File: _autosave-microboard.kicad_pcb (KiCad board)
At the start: 2 copper layers, 95 parts, among them J1 Conn_01x01, J10 Conn_01x01, J11 Conn_01x01, J12 Conn_01x10, J13 Conn_01x01, J17 Conn_01x01, J18 Conn_01x01, J2 Conn_01x10, J21 Conn_01x01_Socket, J22 Conn_01x01_Socket, J24 Conn_01x01, J25 Conn_01x01, J3 Conn_02x12, J39 Conn_01x10, J4 USB_C_Receptacle_USB2.0, J40 Conn_01x10, J41 Conn_01x10, J43 Conn_01x05, J44 Conn_01x09, J45 Conn_01x08, J5 Conn_01x04, J6 Conn_01x04, J7 Conn_01x05, J8 Conn_01x10, J9 Conn_01x01, SW1 SW_Push, SW3 SW_Push, SW4 SW_Push, SW7 RotaryEncoder_Switch, U1 USBLC6-2SC6, U2 ATSAMD21G18A-AUT, U3 LF33_TO220, U4 TXS0108EPW, U7 LF50_TO220, Y1 32768Hz

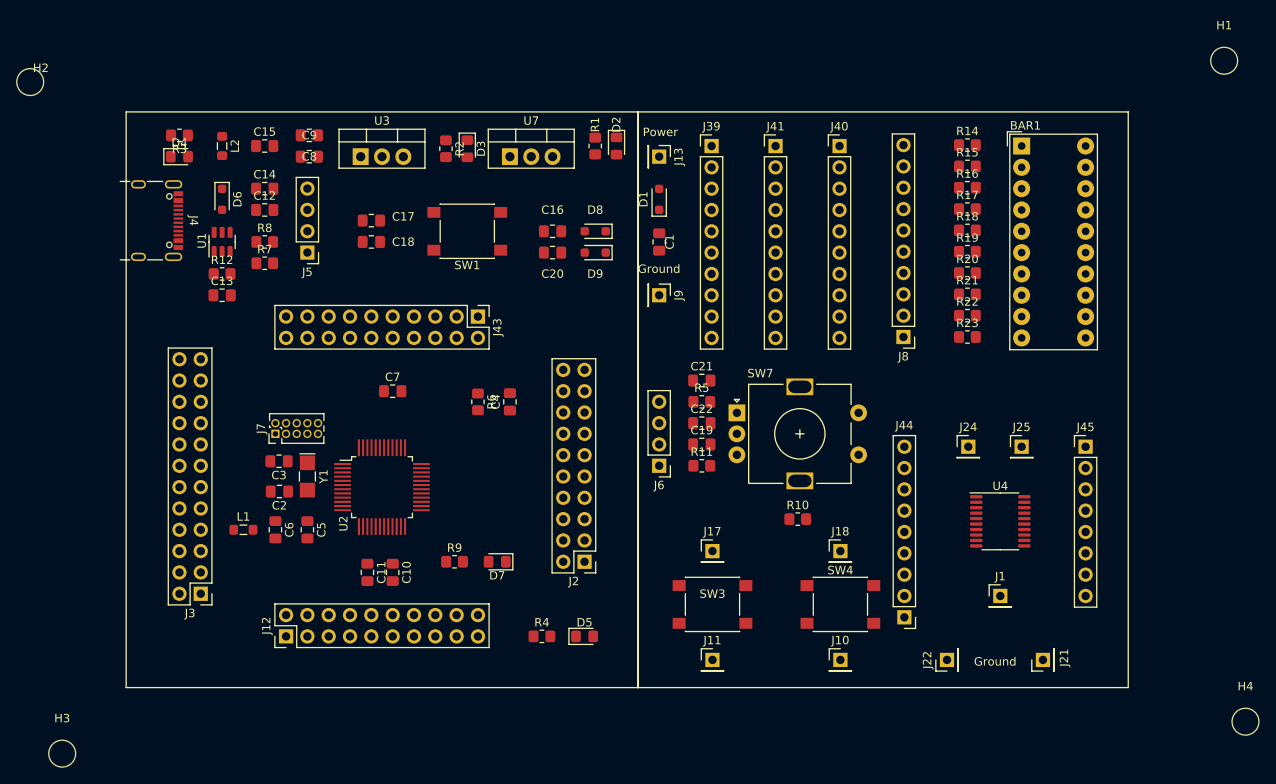
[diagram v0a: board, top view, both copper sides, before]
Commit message: updated
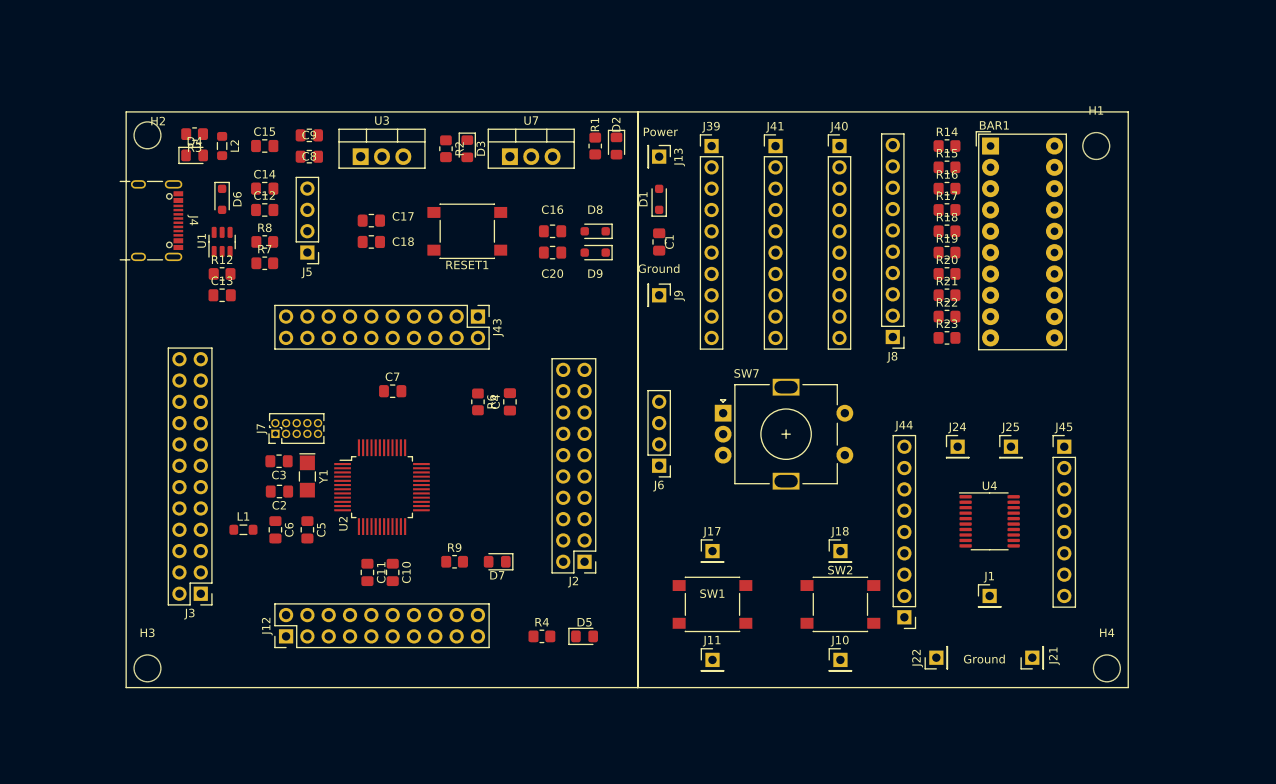
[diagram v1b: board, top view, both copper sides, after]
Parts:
- removed C19, C21, C22: 0.1uF, Capacitor_SMD:C_0805_2012Metric_Pad1.18x1.45mm_HandSolder
- removed R10, R11, R5: 22K, Resistor_SMD:R_0805_2012Metric_Pad1.20x1.40mm_HandSolder
- moved H1 18.3 mm to (242.6, 59.7)
- moved H4 17.7 mm to (243.8, 121.9)
- moved H2 15.3 mm to (129.5, 58.4)
- moved H3 14.4 mm to (129.5, 121.9)
- moved BAR1 3.70 mm to (230.0, 59.7)
- moved J45 2.54 mm to (238.8, 95.5)
- moved R14 2.43 mm to (224.8, 59.7)
- moved R15 2.43 mm to (224.8, 62.2)
- moved R16 2.43 mm to (224.8, 64.8)
- moved R17 2.43 mm to (224.8, 67.3)
- moved R19 2.43 mm to (224.8, 72.4)
- moved R20 2.43 mm to (224.8, 74.9)
- moved R21 2.43 mm to (224.8, 77.5)
- moved R22 2.43 mm to (224.8, 80.0)
- moved R23 2.43 mm to (224.8, 82.5)
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- renumbered SW1 to RESET1, SW3 to SW1, SW4 to SW2
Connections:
- J12 pad 10: GND -> Net-(J12-Pin_10)
- J12 pad 11: +3.3V -> Net-(J12-Pin_11)
- J12 pad 12: Net-(J12-Pin_12) -> Net-(J12-Pin_11)
- J12 pad 14: Net-(J12-Pin_14) -> Net-(J12-Pin_13)
- J12 pad 16: Net-(J12-Pin_16) -> Net-(J12-Pin_15)
- J12 pad 18: Net-(J12-Pin_18) -> Net-(J12-Pin_17)
- J12 pad 19: Net-(J12-Pin_19) -> GND
- J12 pad 2: Net-(J12-Pin_12) -> +3.3V
- J12 pad 3: Net-(J12-Pin_13) -> Net-(J12-Pin_3)
- J12 pad 4: Net-(J12-Pin_14) -> Net-(J12-Pin_3)
- J12 pad 5: Net-(J12-Pin_15) -> Net-(J12-Pin_5)
- J12 pad 6: Net-(J12-Pin_16) -> Net-(J12-Pin_5)
- J12 pad 7: Net-(J12-Pin_17) -> Net-(J12-Pin_7)
- J12 pad 8: Net-(J12-Pin_18) -> Net-(J12-Pin_7)
- J12 pad 9: Net-(J12-Pin_19) -> Net-(J12-Pin_10)
- J2 pad 10: GND -> Net-(J2-Pin_10)
- J2 pad 11: +3.3V -> Net-(J2-Pin_11)
- J2 pad 12: Net-(J2-Pin_12) -> Net-(J2-Pin_11)
- J2 pad 14: Net-(J2-Pin_14) -> Net-(J2-Pin_13)
- J2 pad 16: Net-(J2-Pin_16) -> Net-(J2-Pin_15)
- J2 pad 18: Net-(J2-Pin_18) -> Net-(J2-Pin_17)
- J2 pad 19: Net-(J2-Pin_19) -> GND
- J2 pad 2: Net-(J2-Pin_12) -> +3.3V
- J2 pad 3: Net-(J2-Pin_13) -> Net-(J2-Pin_3)
- J2 pad 4: Net-(J2-Pin_14) -> Net-(J2-Pin_3)
- J2 pad 5: Net-(J2-Pin_15) -> Net-(J2-Pin_5)
- J2 pad 6: Net-(J2-Pin_16) -> Net-(J2-Pin_5)
- J2 pad 7: Net-(J2-Pin_17) -> Net-(J2-Pin_7)
- J2 pad 8: Net-(J2-Pin_18) -> Net-(J2-Pin_7)
- J2 pad 9: Net-(J2-Pin_19) -> Net-(J2-Pin_10)
- J39 pad 1: Net-(D8-K) -> +3.3V
- J39 pad 10: Net-(D8-K) -> +3.3V
- J39 pad 2: Net-(D8-K) -> +3.3V
- J39 pad 3: Net-(D8-K) -> +3.3V
- J39 pad 4: Net-(D8-K) -> +3.3V
- J39 pad 5: Net-(D8-K) -> +3.3V
- J39 pad 6: Net-(D8-K) -> +3.3V
- J39 pad 7: Net-(D8-K) -> +3.3V
- J39 pad 8: Net-(D8-K) -> +3.3V
- J39 pad 9: Net-(D8-K) -> +3.3V
- J40 pad 1: Net-(D9-K) -> +5V
- J40 pad 10: Net-(D9-K) -> +5V
- J40 pad 2: Net-(D9-K) -> +5V
- J40 pad 3: Net-(D9-K) -> +5V
- J40 pad 4: Net-(D9-K) -> +5V
- J40 pad 5: Net-(D9-K) -> +5V
- J40 pad 6: Net-(D9-K) -> +5V
- J40 pad 7: Net-(D9-K) -> +5V
- J40 pad 8: Net-(D9-K) -> +5V
- J40 pad 9: Net-(D9-K) -> +5V
- J43 pad 10: GND -> Net-(J43-Pin_10)
- J43 pad 11: +3.3V -> Net-(J43-Pin_11)
- J43 pad 12: Net-(J43-Pin_12) -> Net-(J43-Pin_11)
- J43 pad 14: Net-(J43-Pin_14) -> Net-(J43-Pin_13)
- J43 pad 16: Net-(J43-Pin_16) -> Net-(J43-Pin_15)
- J43 pad 17: Net-(J43-Pin_17) -> GND
- J43 pad 18: Net-(J43-Pin_18) -> GND
- J43 pad 2: Net-(J43-Pin_12) -> +3.3V
- J43 pad 3: Net-(J43-Pin_13) -> Net-(J43-Pin_3)
- J43 pad 4: Net-(J43-Pin_14) -> Net-(J43-Pin_3)
- J43 pad 5: Net-(J43-Pin_15) -> Net-(J43-Pin_5)
- J43 pad 6: Net-(J43-Pin_16) -> Net-(J43-Pin_5)
- J43 pad 7: Net-(J43-Pin_17) -> Net-(J43-Pin_7)
- J43 pad 8: Net-(J43-Pin_18) -> Net-(J43-Pin_7)
- J43 pad 9: GND -> Net-(J43-Pin_10)
- J7 pad 1: Net-(J43-Pin_18) -> Net-(J43-Pin_15)
- J7 pad 2: Net-(J43-Pin_17) -> Net-(J43-Pin_13)
- SW7 pad A: Net-(R5-Pad2) -> Net-(J6-Pin_3)
- SW7 pad B: Net-(R11-Pad2) -> Net-(J6-Pin_2)
- SW7 pad S1: Net-(R10-Pad2) -> Net-(J6-Pin_4)
- U2 pad 14: Net-(J12-Pin_12) -> Net-(J12-Pin_3)
- U2 pad 15: Net-(J12-Pin_13) -> Net-(J12-Pin_5)
- U2 pad 16: Net-(J12-Pin_14) -> Net-(J12-Pin_7)
- U2 pad 19: Net-(J12-Pin_15) -> Net-(J12-Pin_10)
- U2 pad 20: Net-(J12-Pin_16) -> Net-(J12-Pin_11)
- U2 pad 21: Net-(J12-Pin_17) -> Net-(J12-Pin_13)
- U2 pad 22: Net-(J12-Pin_18) -> Net-(J12-Pin_15)
- U2 pad 23: Net-(J12-Pin_19) -> Net-(J12-Pin_17)
- U2 pad 24: Net-(J2-Pin_12) -> Net-(J2-Pin_3)
- U2 pad 25: Net-(J2-Pin_13) -> Net-(J2-Pin_5)
- U2 pad 26: Net-(J2-Pin_14) -> Net-(J2-Pin_7)
- U2 pad 27: Net-(J2-Pin_15) -> Net-(J2-Pin_10)
- U2 pad 28: Net-(J2-Pin_16) -> Net-(J2-Pin_11)
- U2 pad 29: Net-(J2-Pin_17) -> Net-(J2-Pin_13)
- U2 pad 30: Net-(J2-Pin_18) -> Net-(J2-Pin_15)
- U2 pad 31: Net-(J2-Pin_19) -> Net-(J2-Pin_17)
- U2 pad 32: Net-(J43-Pin_12) -> Net-(J43-Pin_3)
- U2 pad 37: Net-(J43-Pin_13) -> Net-(J43-Pin_5)
- U2 pad 38: Net-(J43-Pin_14) -> Net-(J43-Pin_7)
- U2 pad 39: Net-(J43-Pin_15) -> Net-(J43-Pin_10)
- U2 pad 41: Net-(J43-Pin_16) -> Net-(J43-Pin_11)
- U2 pad 45: Net-(J43-Pin_17) -> Net-(J43-Pin_13)
- U2 pad 46: Net-(J43-Pin_18) -> Net-(J43-Pin_15)
